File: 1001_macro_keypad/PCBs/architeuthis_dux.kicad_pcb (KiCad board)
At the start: 2 copper layers, 145.7 x 117.9 mm, 43 parts, among them J1 ePaperModule, J2 RotaryModule_01, J3 RotaryModule_02, SW01 MX_SW, SW10 MX_SW, SW11 MX_SW, SW12 MX_SW, SW13 MX_SW, SW14 MX_SW, SW2 MX_SW, SW3 MX_SW, SW4 MX_SW, SW5 MX_SW, SW6 MX_SW, SW7 MX_SW, SW8 MX_SW, SW9 MX_SW, U1 Pico

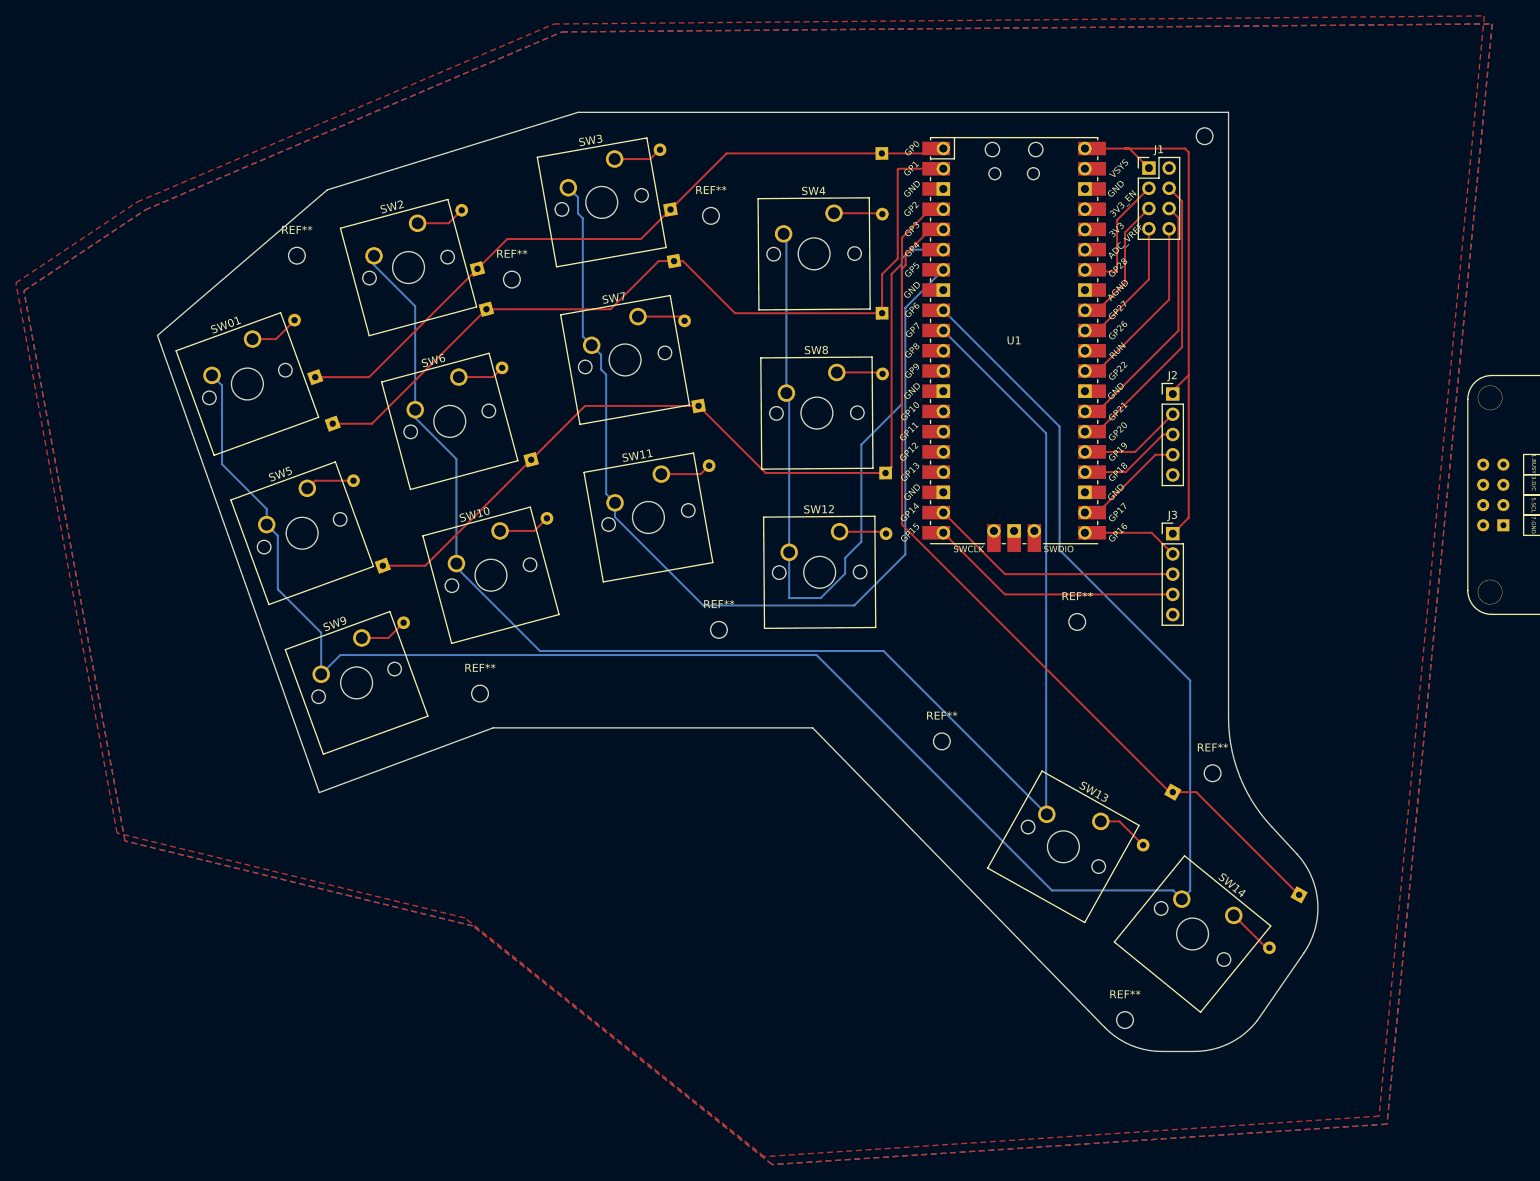
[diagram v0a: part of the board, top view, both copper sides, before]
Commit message: pcb 완성, 3d모델 시작
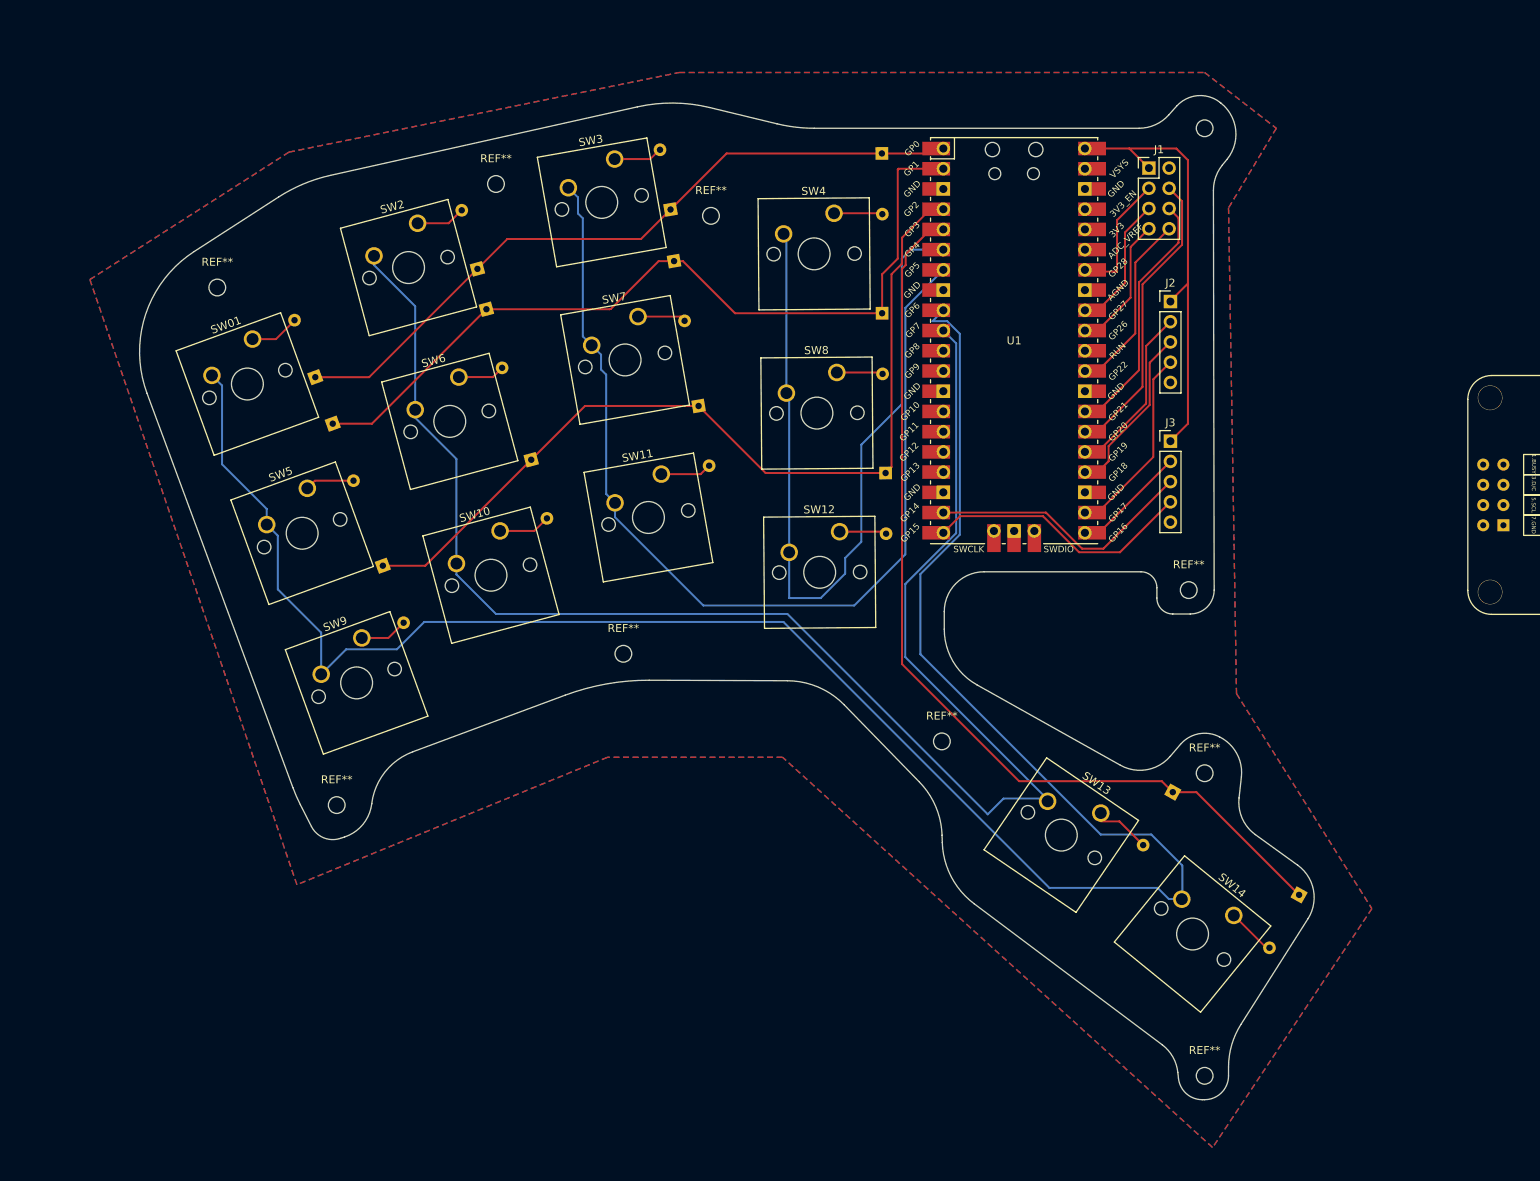
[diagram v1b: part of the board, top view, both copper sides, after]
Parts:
- moved REF** 22.8 mm to (149.0, 124.0)
- moved REF** 14.6 mm to (256.0, 97.0)
- moved REF** 12.4 mm to (185.0, 105.0)
- moved REF** 12.2 mm to (258.0, 158.0)
- moved REF** 12.2 mm to (169.0, 46.0)
- moved J3 11.6 mm to (253.7, 78.3)
- moved J2 11.6 mm to (253.7, 60.8)
- moved REF** 10.8 mm to (134.0, 59.0)
- moved SW13 1.05 mm to (245.0, 125.0), turned to -34.25 degrees
- moved REF** 1.00 mm to (258.0, 120.0)
- moved REF** 1.00 mm to (258.0, 39.0)
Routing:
- net +5V: track 70.0 -> 56.4 mm
- net COL2: track 252.2 -> 264.9 mm
- net ROW3: track 109.3 -> 119.5 mm
- net Net-(J2-S1): track 14.0 -> 24.3 mm
- net Net-(J2-S2): track 13.0 -> 21.7 mm
- net Net-(J2-KEY): track 13.0 -> 21.7 mm
- net COL3: track 196.5 -> 201.2 mm
- net Net-(J3-Pin_2): track 12.1 -> 14.5 mm
- net Net-(J3-Pin_3): track 32.0 -> 33.9 mm
- net Net-(J3-Pin_4): track 32.3 -> 33.9 mm
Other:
- board size 145.7 x 117.9 mm -> 147.5 x 126.1 mm
